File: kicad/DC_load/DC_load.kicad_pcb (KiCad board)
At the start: 2 copper layers, 110 x 145 mm, 155 parts, among them J1 BNC, J2 red_terminal, J3 red terminal, J4 black terminal, J5 black terminal, J6 USB_B, J8 Conn_01x05_Socket, J9 Conn_01x04_Socket, Q1 MMBT5401, Q3 FQP19N20C, Q4 FQP19N20C, Q5 FQP19N20C, Q6 FQP19N20C, SW1 RotaryEncoder_Switch, SW2 RotaryEncoder_Switch, SW3 SW_Push, SW8 SW_Push, U1 FSA3157P6X, U10 FSA3157P6X, U11 FSA3157P6X, U12 FSA3157P6X, U13 TLV9062, U14 AMS1117-3.3, U15 74HC14D653, U17 CH340C, U18 TL431DBZ, U2 Screen, U3 NCS21802, U4 NCS21802, U5 TLV9062, U6 TLV9062, U7 LMT84LPM, U8 STM32F103C8Tx, U9 Front plate

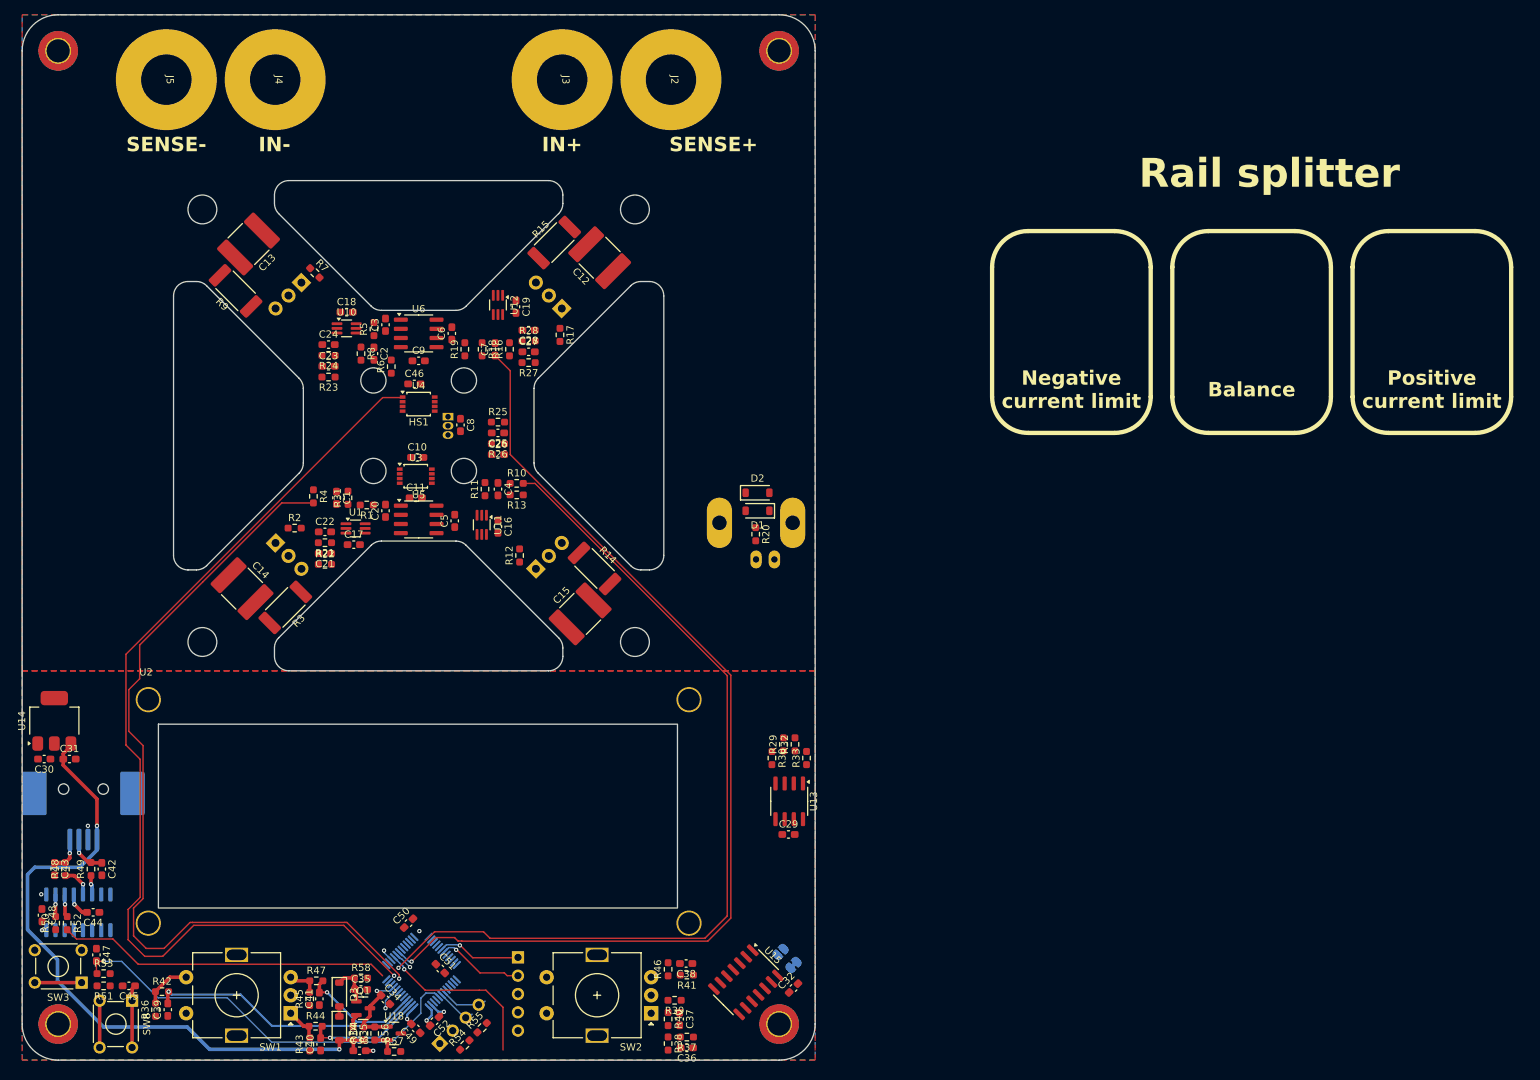
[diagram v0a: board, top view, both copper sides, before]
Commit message: Compressed.
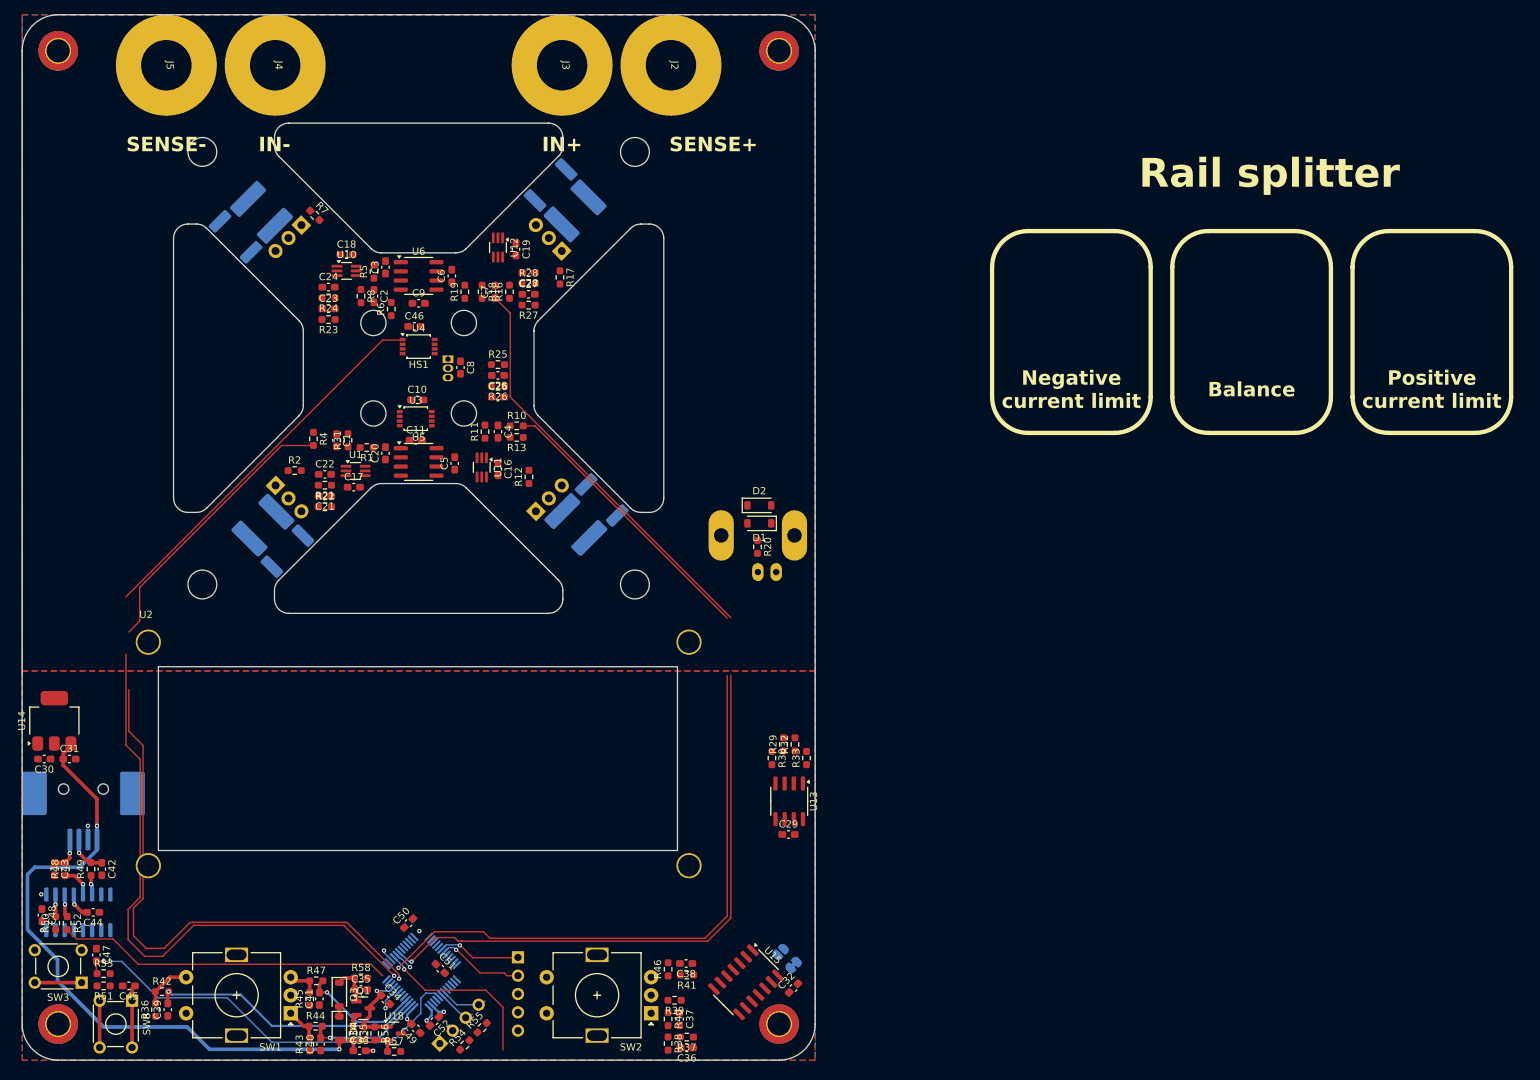
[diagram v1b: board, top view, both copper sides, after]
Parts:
- C12, C13, C14, C15, R14, R15, R3, R9: moved to B.Cu
- moved C15 12.4 mm to (126.8, 120.7), turned to -45 degrees
- moved R12 11.0 mm to (120.3, 114.1)
- moved R14 9.55 mm to (130.4, 117.3)
- moved C14 9.27 mm to (83.4, 120.8), turned to -135 degrees
- moved R15 8.02 mm to (123.3, 73.6)
- moved C1 7.98 mm to (93.6, 109.0)
- moved C10 7.98 mm to (104.8, 103.4)
- moved C11 7.98 mm to (104.6, 109.0)
- moved C16 7.98 mm to (116.0, 113.0)
- moved C17 7.98 mm to (96.0, 115.5)
- moved C18 7.98 mm to (95.0, 83.3)
- moved C19 7.98 mm to (118.5, 82.5)
- moved C2 7.98 mm to (98.8, 89.0)
- moved C21 7.98 mm to (92.0, 116.8)
- moved C22 7.98 mm to (92.0, 113.8)
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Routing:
- net /Microcontroller/CH1_MEAS: track 117.2 -> 39.1 mm
- net /Microcontroller/CH2_MEAS: track 136.9 -> 215.1 mm
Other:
- board text added: "NO THERMAL PADS; VIN needs no polygon"
